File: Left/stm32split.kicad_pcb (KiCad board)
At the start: 2 copper layers, 152.4 x 110.3 mm, 88 parts, among them J1 Conn_01x04, SW1 SW_Push, SW10 SW_Push, SW11 SW_Push, SW12 SW_Push, SW13 SW_Push, SW14 SW_Push, SW15 SW_Push, SW16 SW_Push, SW17 SW_Push, SW18 SW_Push, SW19 SW_Push, SW2 SW_Push, SW20 SW_Push, SW21 SW_Push, SW22 SW_Push, SW23 SW_Push, SW24 SW_Push, SW25 SW_Push, SW26 SW_Push, SW27 SW_Push, SW28 SW_Push, SW29 SW_Push, SW3 SW_Push, SW30 SW_Push, SW31 SW_Push, SW4 SW_Push, SW5 SW_Push, SW6 SW_Push, SW7 SW_Push, SW8 SW_Push, SW9 SW_Push, U1 SRV05-4, U2 STM32F103CBTx, U3 XC6206PxxxMR, Y1 8MHz

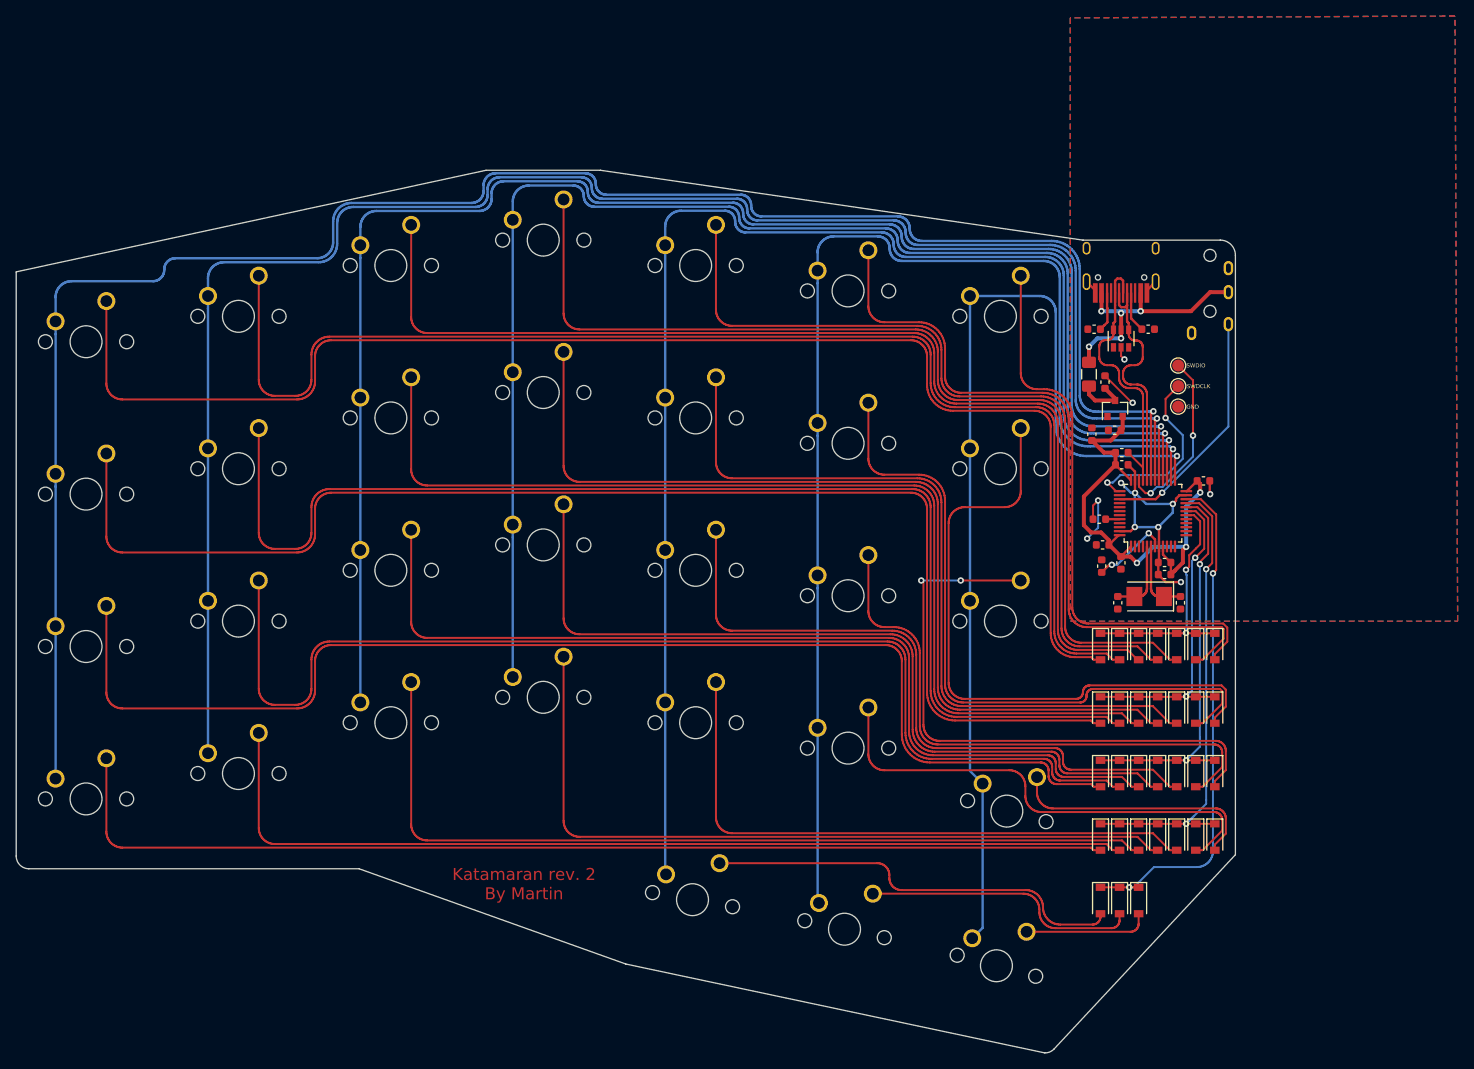
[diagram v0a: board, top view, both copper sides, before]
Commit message: rev2
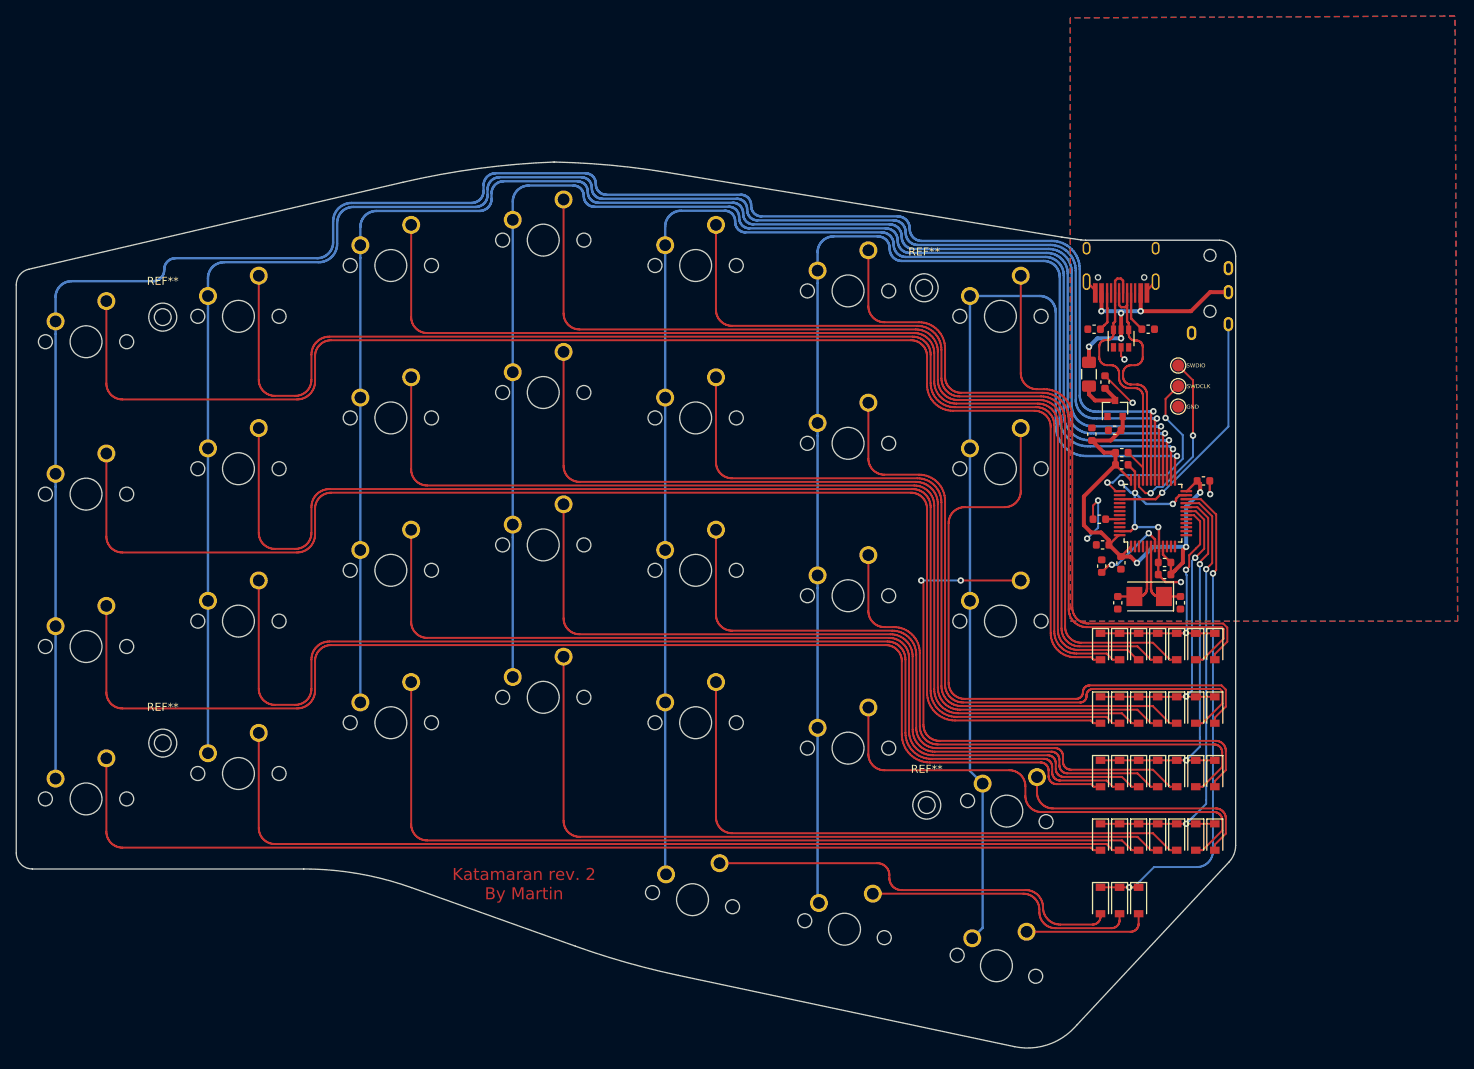
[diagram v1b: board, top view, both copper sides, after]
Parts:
- added REF**: MountingHole_3.5mm, MountingHole:MountingHole_3.5mm, F.Cu at (167.0, 150.0)
- added REF**: MountingHole_3.5mm, MountingHole:MountingHole_3.5mm, F.Cu at (71.5, 142.2)
- added REF**: MountingHole_3.5mm, MountingHole:MountingHole_3.5mm, F.Cu at (71.5, 89.0)
- added REF**: MountingHole_3.5mm, MountingHole:MountingHole_3.5mm, F.Cu at (166.7, 85.3)
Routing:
- net GND: track 55.8 -> 52.1 mm
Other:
- board size 152.4 x 110.3 mm -> 152.4 x 110.7 mm
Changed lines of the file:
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@@
-(kicad_pcb (version 20171130) (host pcbnew "(5.1.4-0)")
+(kicad_pcb (version 20171130) (host pcbnew "(5.1.4)-1")
   (general
     (thickness 1.6)
-    (drawings 239)
-    (tracks 3846)
+    (drawings 251)
+    (tracks 3844)
     (zones 0)
-    (modules 88)
+    (modules 92)
     (nets 82)
   )
@@
     (39 F.Mask user)
     (40 Dwgs.User user)
-    (41 Cmts.User user)
+    (41 Cmts.User user hide)
     (42 Eco1.User user hide)
     (43 Eco2.User user hide)
     (44 Edge.Cuts user)
-    (45 Margin user hide)
-    (46 B.CrtYd user hide)
-    (47 F.CrtYd user hide)
-    (48 B.Fab user hide)
-    (49 F.Fab user hide)
+    (45 Margin user)
+    (46 B.CrtYd user)
+    (47 F.CrtYd user)
+    (48 B.Fab user)
+    (49 F.Fab user)
   )
   (setup
@@
     (solder_mask_min_width 0.25)
     (aux_axis_origin 0 0)
-    (visible_elements FFFFFF7F)
+    (visible_elements 7FFFFFFF)
     (pcbplotparams
-      (layerselection 0x010fc_ffffffff)
+      (layerselection 0x290fc_ffffffff)
       (usegerberextensions false)
       (usegerberattributes false)
@@
       (drillshape 0)
       (scaleselection 1)
-      (outputdirectory ""))
+      (outputdirectory "gerber"))
   )
   (net 0 "")
@@
     (add_net VBUS)
   )
+  (module MountingHole:MountingHole_3.5mm (layer F.Cu)
+    (at 167.000002 150.000002)
+    (descr "Mounting Hole 3.5mm, no annular")
+    (tags "mounting hole 3.5mm no annular")
+    (attr virtual)
+    (fp_text reference REF** (at 0 -4.5) (layer F.SilkS)
+      (effects (font (size 1 1) (thickness 0.15)))
+    )
+    (fp_text value MountingHole_3.5mm (at 0 4.5) (layer F.Fab)
+      (effects (font (size 1 1) (thickness 0.15)))
+    )
+    (fp_circle (center 0 0) (end 3.75 0) (layer F.CrtYd) (width 0.05))
+    (fp_circle (center 0 0) (end 3.5 0) (layer Cmts.User) (width 0.15))
+    (fp_text user %R (at 0.3 0) (layer F.Fab)
+      (effects (font (size 1 1) (thickness 0.15)))
+    )
+    (pad 1 np_thru_hole circle (at 0 0) (size 3.5 3.5) (drill 3.5) (layers *.Cu *.Mask))
+  )
+  (module MountingHole:MountingHole_3.5mm (layer F.Cu)
+    (at 71.502024 142.247519)
+    (descr "Mounting Hole 3.5mm, no annular")
+    (tags "mounting hole 3.5mm no annular")
+    (attr virtual)
+    (fp_text reference REF** (at 0 -4.5) (layer F.SilkS)
+      (effects (font (size 1 1) (thickness 0.15)))
+    )
+    (fp_text value MountingHole_3.5mm (at 0 4.5) (layer F.Fab)
+      (effects (font (size 1 1) (thickness 0.15)))
+    )
+    (fp_circle (center 0 0) (end 3.75 0) (layer F.CrtYd) (width 0.05))
+    (fp_circle (center 0 0) (end 3.5 0) (layer Cmts.User) (width 0.15))
+    (fp_text user %R (at 0.3 0) (layer F.Fab)
+      (effects (font (size 1 1) (thickness 0.15)))
+    )
+    (pad 1 np_thru_hole circle (at 0 0) (size 3.5 3.5) (drill 3.5) (layers *.Cu *.Mask))
+  )
+  (module MountingHole:MountingHole_3.5mm (layer F.Cu)
+    (at 71.500001 89.000001)
+    (descr "Mounting Hole 3.5mm, no annular")
+    (tags "mounting hole 3.5mm no annular")
+    (attr virtual)
+    (fp_text reference REF** (at 0 -4.5) (layer F.SilkS)
+      (effects (font (size 1 1) (thickness 0.15)))
+    )
+    (fp_text value MountingHole_3.5mm (at 0 4.5) (layer F.Fab)
+      (effects (font (size 1 1) (thickness 0.15)))
+    )
+    (fp_circle (center 0 0) (end 3.75 0) (layer F.CrtYd) (width 0.05))
+    (fp_circle (center 0 0) (end 3.5 0) (layer Cmts.User) (width 0.15))
+    (fp_text user %R (at 0.3 0) (layer F.Fab)
+      (effects (font (size 1 1) (thickness 0.15)))
+    )
+    (pad 1 np_thru_hole circle (at 0 0) (size 3.5 3.5) (drill 3.5) (layers *.Cu *.Mask))
+  )
+  (module MountingHole:MountingHole_3.5mm (layer F.Cu)
+    (at 166.673089 85.332471)
+    (descr "Mounting Hole 3.5mm, no annular")
+    (tags "mounting hole 3.5mm no annular")
+    (attr virtual)
+    (fp_text reference REF** (at 0 -4.5) (layer F.SilkS)
+      (effects (font (size 1 1) (thickness 0.15)))
+    )
+    (fp_text value MountingHole_3.5mm (at 0 4.5) (layer F.Fab)
+      (effects (font (size 1 1) (thickness 0.15)))
+    )
+    (fp_circle (center 0 0) (end 3.75 0) (layer F.CrtYd) (width 0.05))
+    (fp_circle (center 0 0) (end 3.5 0) (layer Cmts.User) (width 0.15))
+    (fp_text user %R (at 0.3 0) (layer F.Fab)
+      (effects (font (size 1 1) (thickness 0.15)))
+    )
+    (pad 1 np_thru_hole circle (at 0 0) (size 3.5 3.5) (drill 3.5) (layers *.Cu *.Mask))
+  )
   (module Diode_SMD:D_SOD-123 (layer F.Cu)
     (at 193.485 161.925 270)
@@
     )
   )
+  (gr_circle (center 167.000002 150.000002) (end 168.050002 150.000002) (layer Edge.Cuts) (width 0.05))
+  (gr_circle (center 71.502024 142.247519) (end 72.552024 142.247519) (layer Edge.Cuts) (width 0.05))
+  (gr_circle (center 71.500001 89.000001) (end 72.550001 89.000001) (layer Edge.Cuts) (width 0.05))
+  (gr_circle (center 166.673089 85.332471) (end 167.723089 85.332471) (layer Edge.Cuts) (width 0.05))
+  (gr_line (start 185.470978 177.803027) (end 185.805309 177.444855) (layer Edge.Cuts) (width 0.05))
+  (gr_arc (start 156.716807 73.458994) (end 123.079986 167.632049) (angle -7.679627376) (layer Edge.Cuts) (width 0.05))
+  (gr_line (start 89.128603 157.980256) (end 55.18849 157.980256) (layer Edge.Cuts) (width 0.05))
+  (gr_line (start 53.18849 155.980256) (end 53.18849 84.969599) (layer Edge.Cuts) (width 0.05))
+  (gr_line (start 101.532511 72.140555) (end 54.765824 83.014771) (layer Edge.Cuts) (width 0.05))
+  (gr_arc (start 124.179899 169.542279) (end 120.415741 69.613148) (angle -10.93234955) (layer Edge.Cuts) (width 0.05))
+  (gr_arc (start 118.361726 169.592051) (end 134.541415 70.909643) (angle -8.134262868) (layer Edge.Cuts) (width 0.05))
+  (gr_line (start 183.917346 79.005181) (end 134.541415 70.909643) (layer Edge.Cuts) (width 0.05))
+  (gr_arc (start 55.18849 84.969599) (end 54.765824 83.014771) (angle -77.79953127) (layer Edge.Cuts) (width 0.05))
+  (gr_arc (start 55.18849 155.980256) (end 53.18849 155.980256) (angle -90) (layer Edge.Cuts) (width 0.05))
+  (gr_arc (start 89.128603 197.980256) (end 102.583331 160.311034) (angle -19.65575982) (layer Edge.Cuts) (width 0.05))
+  (gr_line (start 123.079986 167.632049) (end 102.583331 160.311034) (layer Edge.Cuts) (width 0.05))
+  (gr_line (start 177.946709 180.187324) (end 135.966386 171.282407) (layer Edge.Cuts) (width 0.05))
+  (gr_arc (start 179.606743 172.361451) (end 177.946709 180.187324) (angle -59.117092) (layer Edge.Cuts) (width 0.05))
+  (gr_arc (start 186.862245 75.187702) (end 186.260533 79.344376) (angle -8.236800797) (layer Edge.Cuts) (width 0.05))
+  (gr_line (start 186.862245 79.387702) (end 203.612878 79.387702) (layer Edge.Cuts) (width 0.05))
+  (gr_arc (start 203.612878 81.387702) (end 205.612878 81.387702) (angle -90) (layer Edge.Cuts) (width 0.05))
+  (gr_line (start 185.805309 177.444855) (end 204.805929 157.089326) (layer Edge.Cuts) (width 0.05))
+  (gr_arc (start 202.612878 155.042249) (end 204.805929 157.089326) (angle -43.02826554) (layer Edge.Cuts) (width 0.05))
+  (gr_line (start 205.612878 81.387702) (end 205.612878 155.042249) (layer Edge.Cuts) (width 0.05))
+  (gr_line (start 186.260533 79.344376) (end 183.917346 79.005181) (layer Edge.Cuts) (width 0.05))
   (gr_text "Katamaran rev. 2\nBy Martin" (at 116.66 159.87) (layer F.Cu)
     (effects (font (size 1.5 1.5) (thickness 0.3)))
@@
   (gr_line (start 190.54375 87.5075) (end 190.54375 85.9825) (layer F.Mask) (width 0.7))
   (gr_line (start 190.34 90.58) (end 190.34 89.75) (layer F.Mask) (width 0.7))
-  (gr_arc (start 181.76875 179.3875) (end 181.76875 180.975) (angle -45) (layer Edge.Cuts) (width 0.05))
-  (gr_arc (start 203.69375 81.2625) (end 205.58125 81.2625) (angle -90) (layer Edge.Cuts) (width 0.05))
-  (gr_arc (start 54.76875 156.36875) (end 53.18125 156.36875) (angle -90) (layer Edge.Cuts) (width 0.05))
-  (gr_line (start 186.53125 79.375) (end 126.20625 70.64375) (layer Edge.Cuts) (width 0.05))
-  (gr_line (start 111.91875 70.64375) (end 53.18125 83.34375) (layer Edge.Cuts) (width 0.05))
-  (gr_line (start 129.38125 169.8625) (end 96.04375 157.95625) (layer Edge.Cuts) (width 0.05))
-  (gr_line (start 186.53125 79.375) (end 203.69375 79.375) (layer Edge.Cuts) (width 0.05))
-  (gr_line (start 111.91875 70.64375) (end 126.20625 70.64375) (layer Edge.Cuts) (width 0.05))
-  (gr_line (start 53.18125 156.36875) (end 53.18125 83.34375) (layer Edge.Cuts) (width 0.05))
-  (gr_line (start 96.04375 157.95625) (end 54.76875 157.95625) (layer Edge.Cuts) (width 0.05))
-  (gr_line (start 181.76875 180.975) (end 129.38125 169.8625) (layer Edge.Cuts) (width 0.05))
-  (gr_line (start 205.58125 156.2) (end 182.891282 180.510032) (layer Edge.Cuts) (width 0.05))
-  (gr_line (start 205.58125 81.2625) (end 205.58125 156.2) (layer Edge.Cuts) (width 0.05))
   (segment (start 64.4525 97.29) (end 64.4525 86.995) (width 0.25) (layer F.Cu) (net 1))
   (segment (start 64.46213 97.486034) (end 64.4525 97.29) (width 0.25) (layer F.Cu) (net 1))
@@
   (segment (start 193.02 115.25) (end 193.01 115.24) (width 0.3) (layer B.Cu) (net 66))
   (segment (start 195.94 115.25) (end 193.02 115.25) (width 0.3) (layer B.Cu) (net 66))
-  (segment (start 197.76 113.43) (end 197.76 112.35) (width 0.3) (layer B.Cu) (net 66))
-  (segment (start 195.94 115.25) (end 197.76 113.43) (width 0.3) (layer B.Cu) (net 66))
   (segment (start 193.02875 108.32125) (end 192.1675 107.46) (width 0.3) (layer F.Cu) (net 66))
   (segment (start 193.02875 109.34375) (end 193.02875 108.32125) (width 0.3) (layer F.Cu) (net 66))
